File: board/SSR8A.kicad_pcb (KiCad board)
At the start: 2 copper layers, 182 x 48 mm, 35 parts, among them J1 PROG, J2 Conn_01x02, J3 Conn_01x02, J4 Conn_01x02, J5 Conn_01x02, J6 Conn_01x02, J7 Conn_01x02, J8 Conn_01x02, J9 Conn_01x02, U1 HLK-PM01, U10 G3MB-SSR, U11 G3MB-SSR, U2 ESP32-C3-WROOM-02, U3 LM1117-3.3, U4 G3MB-SSR, U5 G3MB-SSR, U6 G3MB-SSR, U7 G3MB-SSR, U8 G3MB-SSR, U9 G3MB-SSR, X1 I2C, X2 I2C, X3 I2C

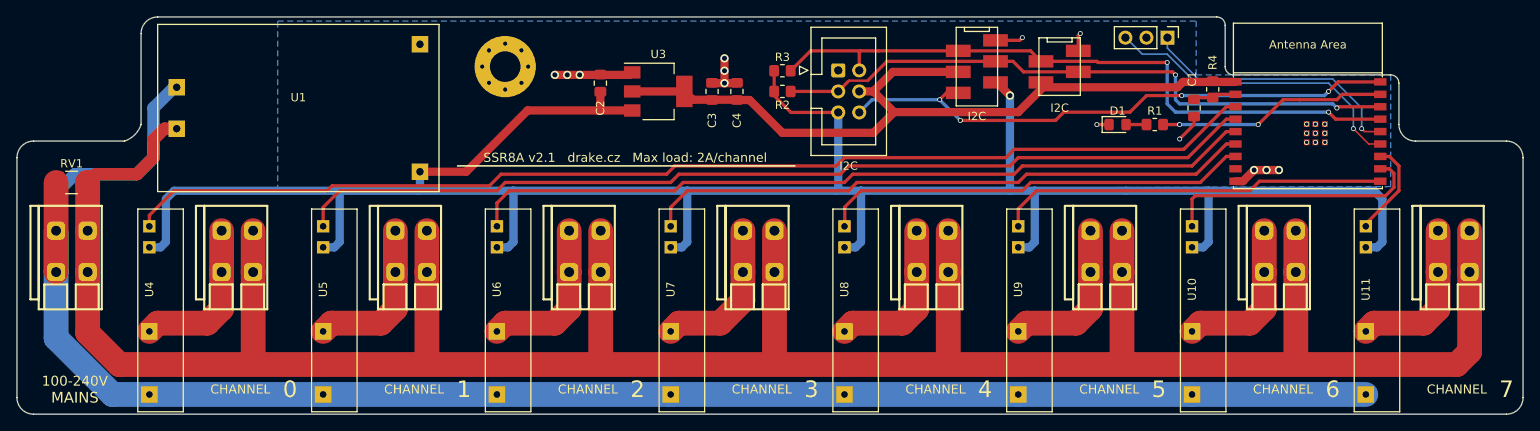
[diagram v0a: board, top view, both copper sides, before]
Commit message: WIP
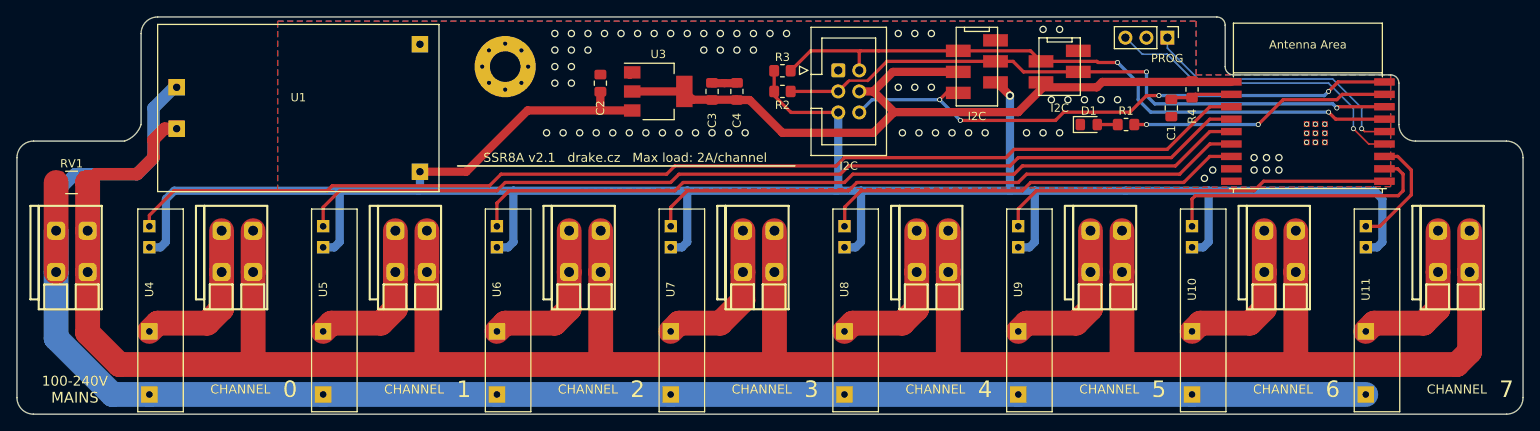
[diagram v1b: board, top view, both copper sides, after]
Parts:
- U2: footprint Espressif:ESP32-C3-WROOM-02 -> Drake:ESP32-C3-WROOM-02 Handsolder
- moved D1 3.47 mm to (179.5, 102.0)
- moved R1 3.47 mm to (184.0, 102.0)
- moved C1 2.75 mm to (189.5, 100.0)
- moved R4 2.50 mm to (192.0, 97.8)
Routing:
- net GND: track 32.2 -> 3.83 mm, vias 22 -> 78
- net /LED: track 27.8 -> 31.7 mm
- net //CH7: track 11.7 -> 14.0 mm
- net Net-(U2-EN/CHIP_PU): track 5.25 -> 7.50 mm
- net //CH6: track 31.9 -> 33.7 mm
- net /SCL: track 81.0 -> 79.7 mm
- net //CH5: track 47.2 -> 47.7 mm
- net //CH4: track 52.1 -> 51.6 mm
- net //CH2: track 95.6 -> 95.1 mm
- net //CH1: track 116.9 -> 116.4 mm
- net /USB_D-: track 37.6 -> 38.1 mm
- net /USB_D+: track 32.6 -> 33.1 mm
- net /ALERT: track 69.2 -> 69.7 mm
- added copper zone on F.Cu, net GND
